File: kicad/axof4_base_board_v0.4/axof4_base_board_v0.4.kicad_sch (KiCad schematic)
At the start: 7 parts, among them J25 SWD, J26 Conn_01x28_Female, J27 Conn_01x24_Female, J28 Conn_01x24_Female, SW5 BOOT_FLASH

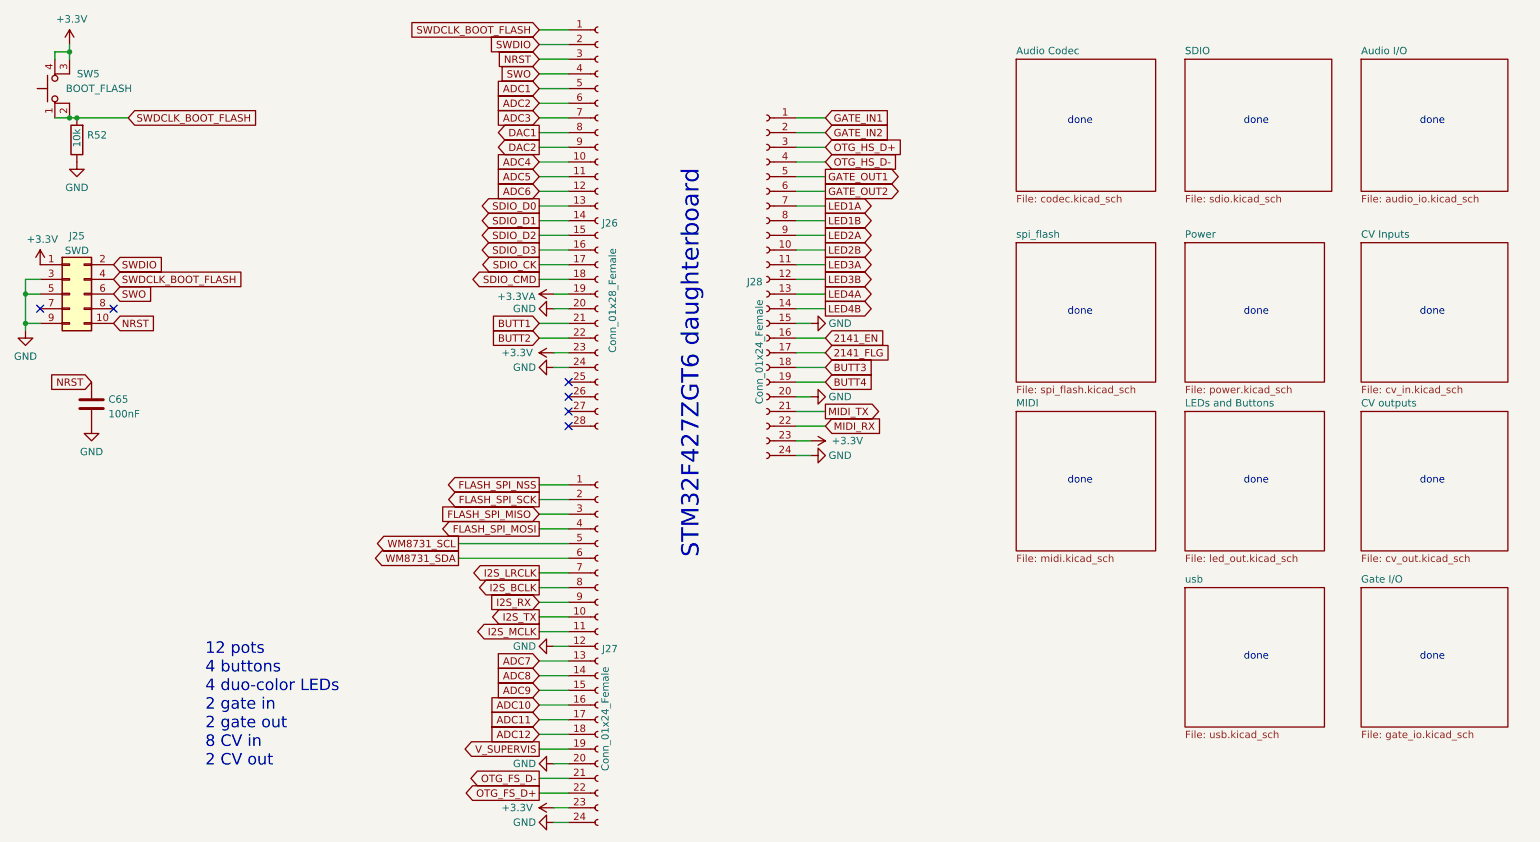
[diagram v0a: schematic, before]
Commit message: revision 4
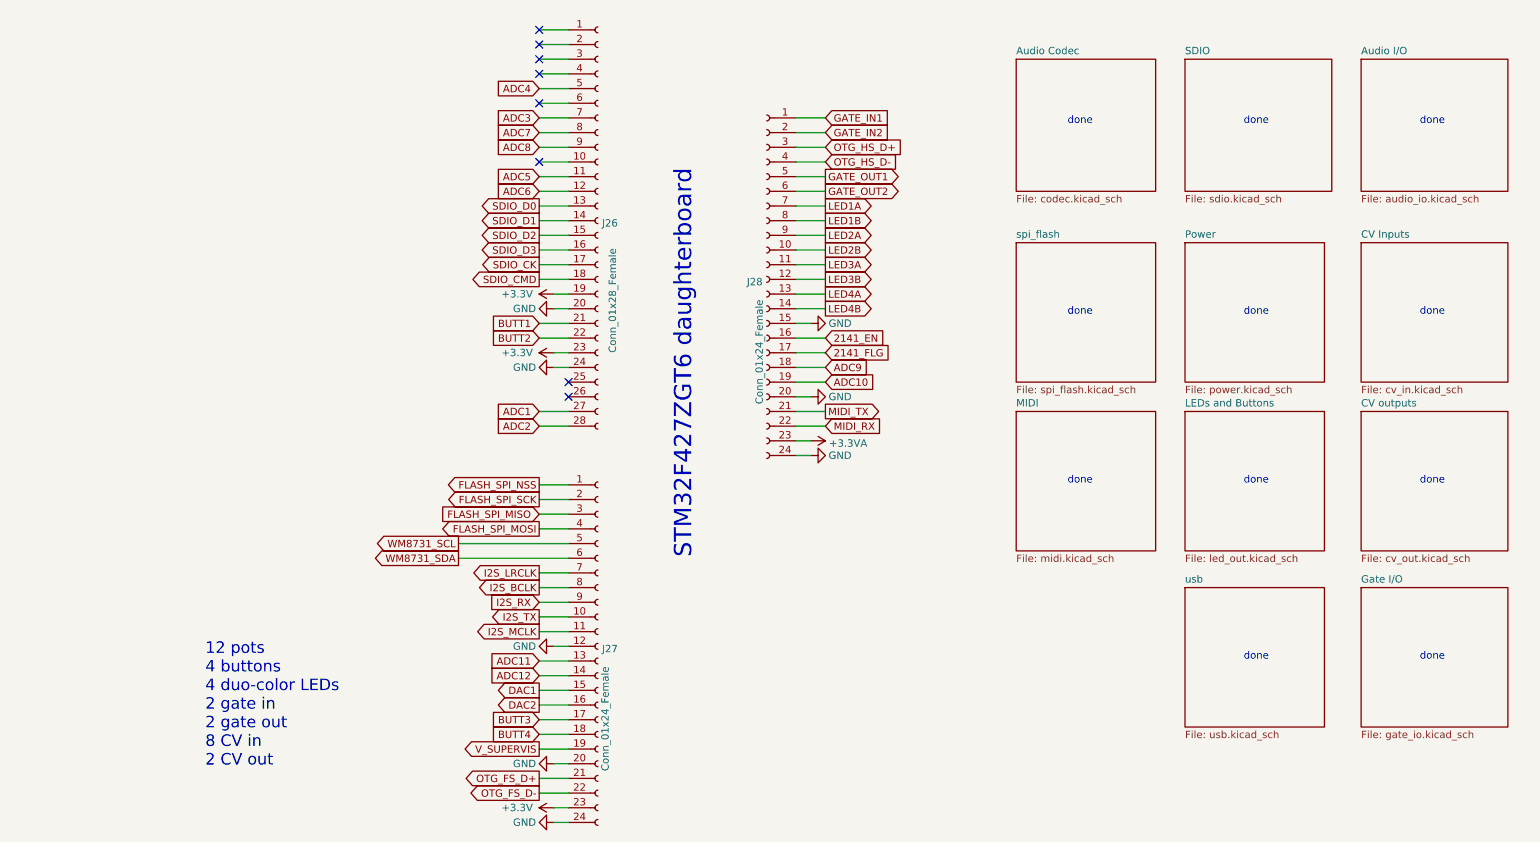
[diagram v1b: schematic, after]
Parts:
- removed C65: 100nF, Capacitor_SMD:C_0603_1608Metric, symbol Device:C
- removed J25: SWD, Connector_PinHeader_1.27mm:PinHeader_2x05_P1.27mm_Vertical_SMD, symbol Connector_Generic:Conn_02x05_Odd_Even
- removed R52: 10k, Resistor_SMD:R_0603_1608Metric, symbol Device:R
- removed SW5: BOOT_FLASH, foots:tactile_TS-1187A, symbol Switch:SW_MEC_5E
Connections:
- net +3.3VA: now also J28.23 (Pin_23); no longer J26.19 (Pin_19)
- net +3V3: now also J26.19 (Pin_19); no longer J28.23 (Pin_23)
- net ADC1: now also J26.27 (Pin_27); no longer J26.5 (Pin_5)
- net ADC10: now also J28.19 (Pin_19); no longer J27.16 (Pin_16)
- net ADC11: now also J27.13 (Pin_13); no longer J27.17 (Pin_17)
- net ADC12: now also J27.14 (Pin_14); no longer J27.18 (Pin_18)
- net ADC2: now also J26.28 (Pin_28); no longer J26.6 (Pin_6)
- net ADC4: now also J26.5 (Pin_5); no longer J26.10 (Pin_10)
- net ADC7: now also J26.8 (Pin_8); no longer J27.13 (Pin_13)
- net ADC8: now also J26.9 (Pin_9); no longer J27.14 (Pin_14)
- net ADC9: now also J28.18 (Pin_18); no longer J27.15 (Pin_15)
- net BUTT3: now also J27.17 (Pin_17); no longer J28.18 (Pin_18)
- net BUTT4: now also J27.18 (Pin_18); no longer J28.19 (Pin_19)
- net DAC1: now also J27.15 (Pin_15); no longer J26.8 (Pin_8)
- net DAC2: now also J27.16 (Pin_16); no longer J26.9 (Pin_9)
- net OTG_FS_D+: now also J27.21 (Pin_21); no longer J27.22 (Pin_22)
- net OTG_FS_D-: now also J27.22 (Pin_22); no longer J27.21 (Pin_21)
- net NRST: no longer names the net of J26.3 (Pin_3)
- net SWDCLK_BOOT_FLASH: no longer names the net of J26.1 (Pin_1)
- net SWDIO: no longer names the net of J26.2 (Pin_2)
- net SWO: no longer names the net of J26.4 (Pin_4)
- no-connect marks 6 -> 8
